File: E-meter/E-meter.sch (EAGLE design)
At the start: 17 parts, among them IC1 LM324N

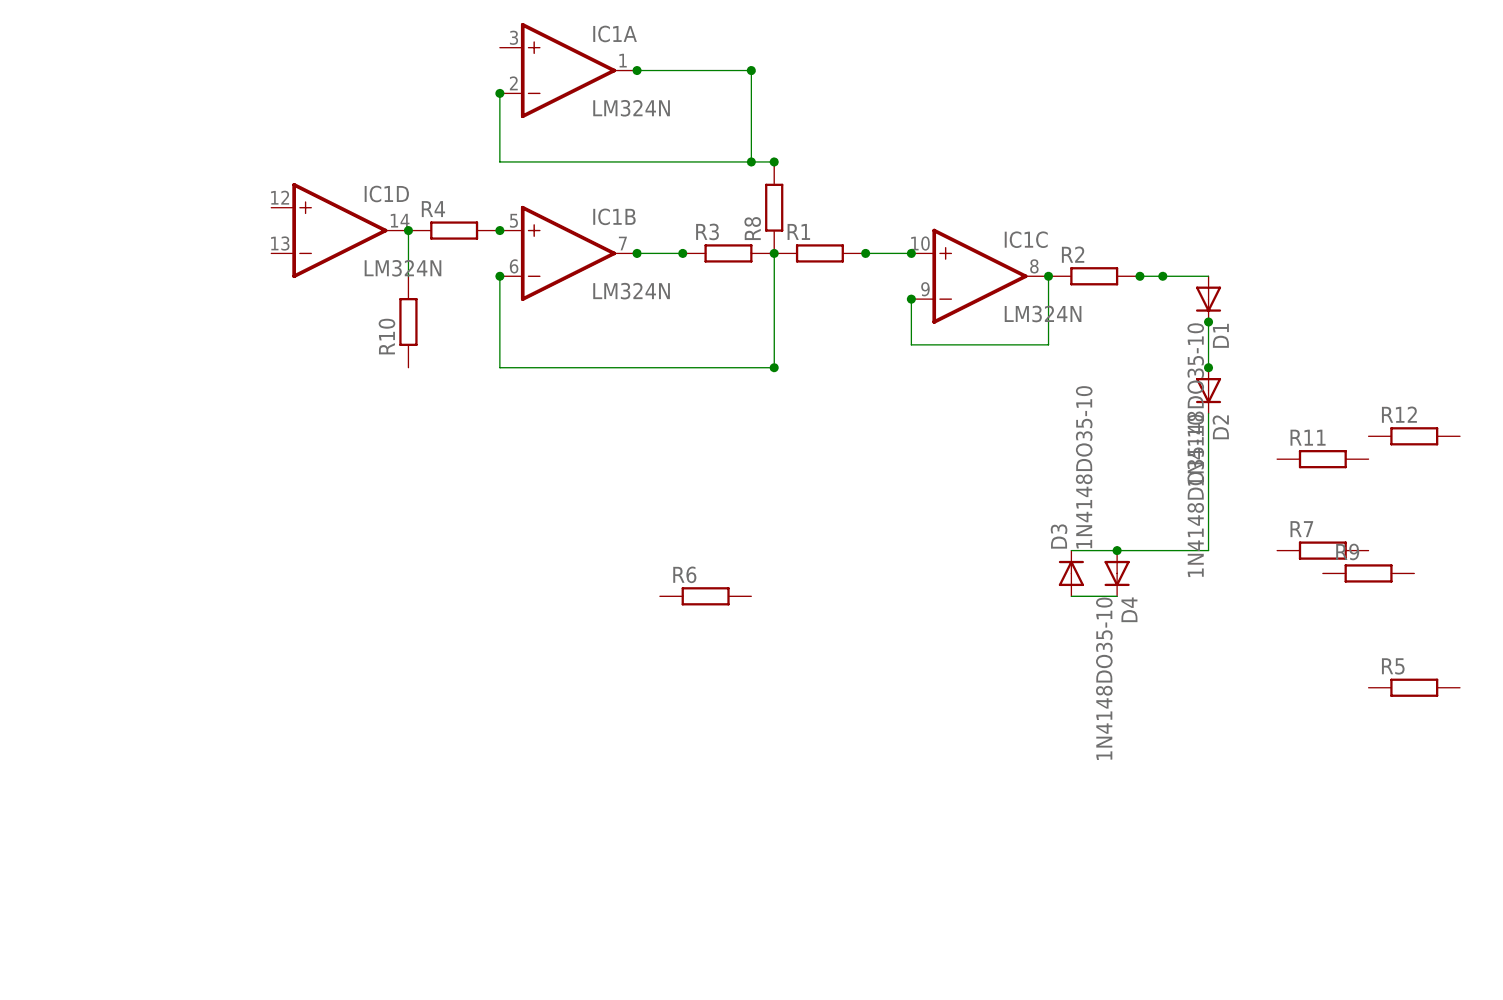
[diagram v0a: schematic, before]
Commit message: First version
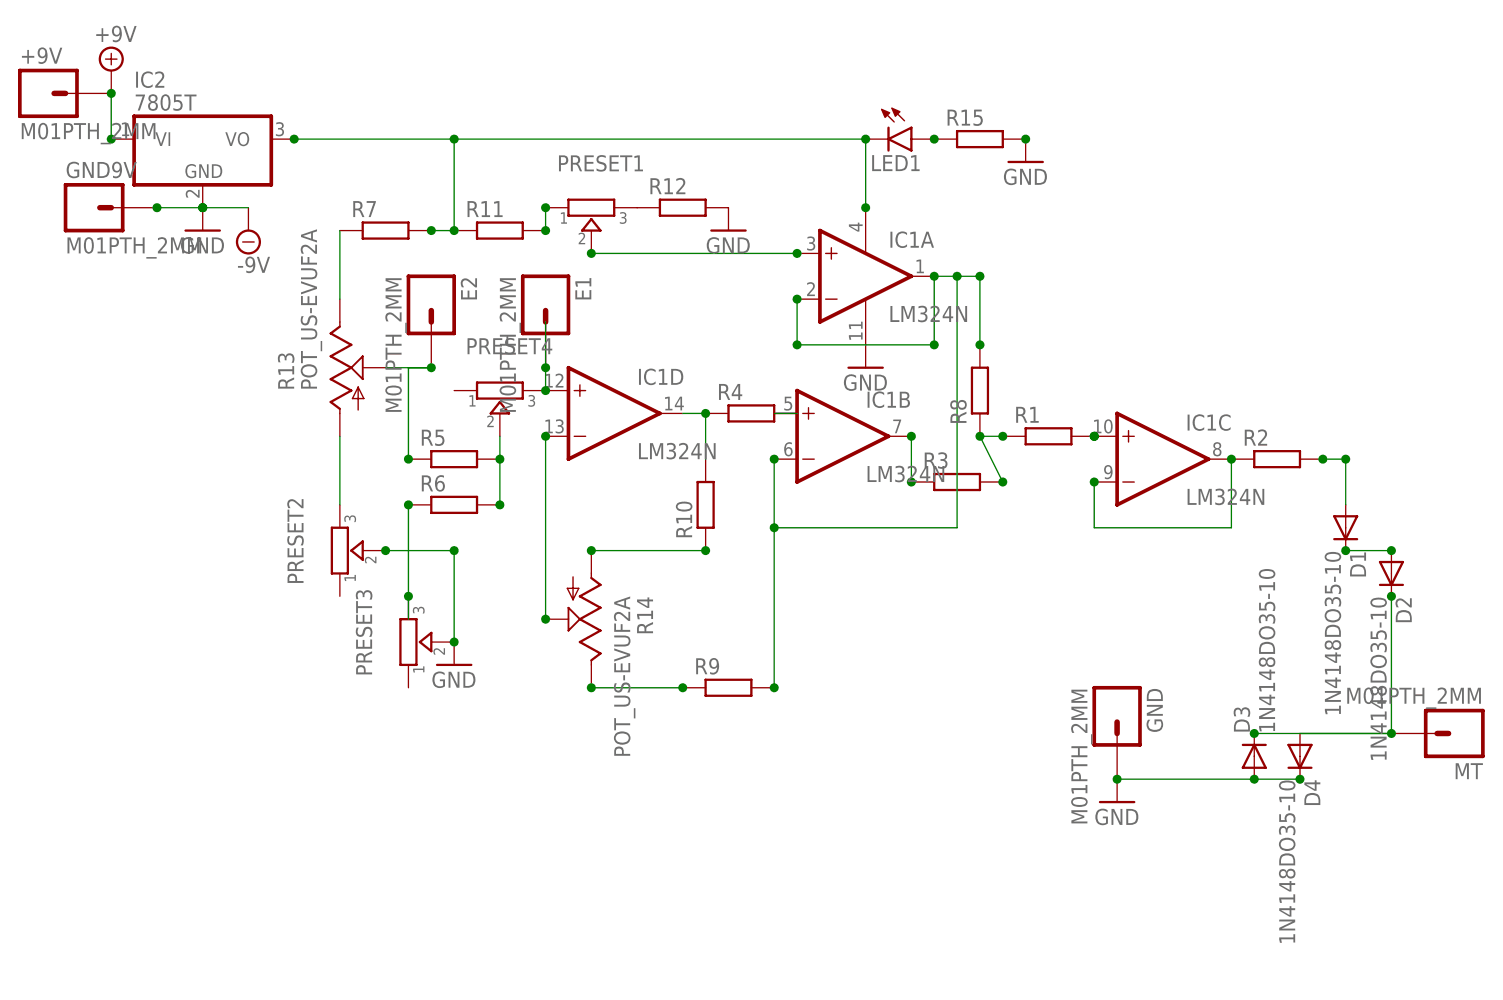
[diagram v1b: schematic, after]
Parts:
- added +9V, E1, E2, GND, GND9V, MT: M01PTH_2MM, SparkFun-Connectors:M01PTH_2MM
- added IC2: 7805T, linear:7805T
- added LED1: (no value), SparkFun-LED:LED5MM
- added PRESET1, PRESET2, PRESET3, PRESET4: (no value), dp_devices:TRIMMER-3306F
- added R13, R14: POT_US-EVUF2A, 4009dist_PWM3_v1:POT_US-EVUF2A
- added R15: (no value), rcl:R-EU_0207/10
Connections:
- new net +9V: +9V.1, IC2.VI
- new net GND: D3.A, D4.C, GND.1, GND9V.1, IC1P.V-, IC2.GND, PRESET2.2, PRESET3.2, R12.2, R15.2
- new net N$12: IC1A.+IN, PRESET1.2
- new net N$13: PRESET1.1, R11.2
- new net N$14: IC1P.V+, IC2.VO, LED1.C, R11.1, R7.2
- new net N$15: R13.E, R7.1
- new net N$16: PRESET1.3, R12.1
- new net N$17: R10.1, R14.A
- new net N$19: PRESET2.3, R13.A
- new net N$20: IC1D.-IN, R14.S
- new net N$21: R14.E, R9.1
- new net N$22: R1.1, R3.2, R8.1
- new net N$23: PRESET4.2, R5.2, R6.2
- new net N$24: PRESET3.3, R6.1
- new net N$26: LED1.A, R15.1
- net N$1: now also E2.1, R13.S, R5.1; no longer IC1A.-IN, IC1A.OUT, R8.2
- net N$11: now also D2.C, D3.C, D4.A, MT.1; no longer D3.A, D4.C
- net N$4: now also IC1A.-IN, IC1A.OUT, R8.2, R9.2; no longer R1.1, R3.2, R8.1
- net N$9: now also E1.1, IC1D.+IN, PRESET4.3; no longer D2.C, D3.C, D4.A
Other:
- moved on the sheet: D1, D2, D3, D4, IC1A, IC1B, IC1C, IC1D, R1, R10, R11, R12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
